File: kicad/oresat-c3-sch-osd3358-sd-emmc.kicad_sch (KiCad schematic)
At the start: 45 parts, among them J5 DM3BT-DSF-PEJS, U1 OSD3358-512M-BSM, U8 TCAN330, U9 EMMC+RESET+5.1-COMPATIBLE-BA

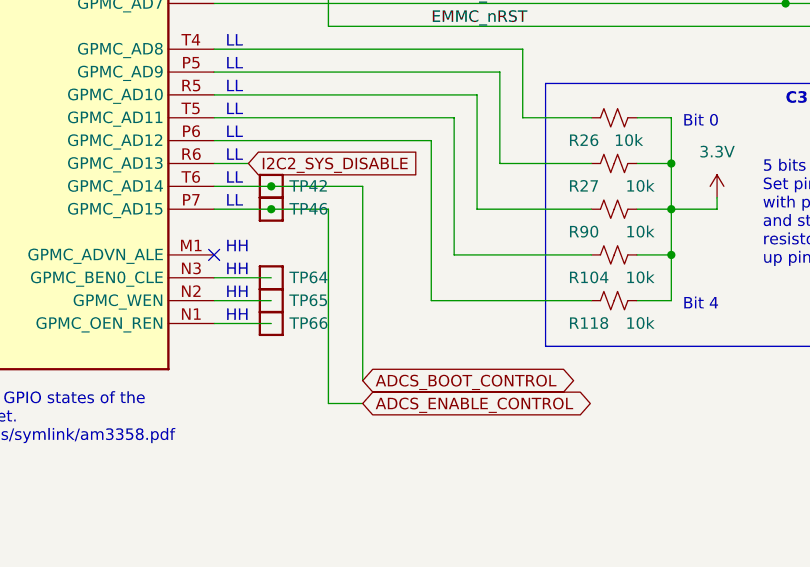
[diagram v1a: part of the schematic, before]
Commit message: - Locked CSKB Headers on PCB - Removed CAN1 from schematic - Removed ADCS boot enable from schematic - Removed unnecessary grounds from PCB
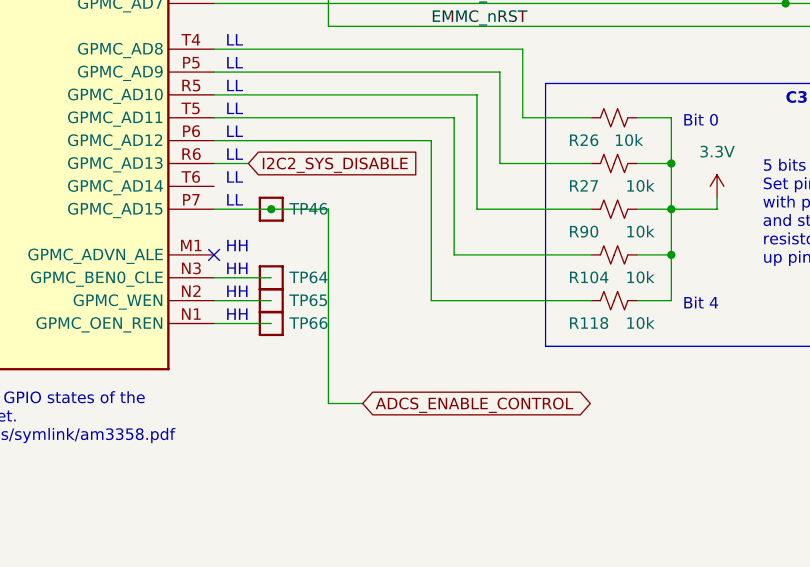
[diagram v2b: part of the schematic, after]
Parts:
- removed TP42: Test-Point, oresat-misc:TestPoint_Pad_D1.0mm, symbol oresat-misc:Test-Point-1mm-round
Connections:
- net ADCS_BOOT_CONTROL: no longer names the net of U1.T6 (GPMC_AD14)
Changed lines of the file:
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@@
 	)
 	(junction
-		(at 229.87 200.66)
-		(diameter 0)
-		(color 0 0 0 0)
-	)
-	(junction
 		(at 269.24 157.48)
 		(diameter 0)
@@
 	(wire
 		(pts
-			(xy 240.03 200.66) (xy 240.03 222.25)
-		)
-		(stroke
-			(width 0)
-			(type default)
-		)
-	)
-	(wire
-		(pts
 			(xy 269.24 104.14) (xy 278.13 104.14)
 		)
@@
 	(wire
 		(pts
-			(xy 240.03 200.66) (xy 229.87 200.66)
-		)
-		(stroke
-			(width 0)
-			(type default)
-		)
-	)
-	(wire
-		(pts
 			(xy 238.76 160.02) (xy 266.7 160.02)
 		)
@@
 	(wire
 		(pts
-			(xy 223.52 200.66) (xy 229.87 200.66)
-		)
-		(stroke
-			(width 0)
-			(type default)
-		)
-	)
-	(wire
-		(pts
 			(xy 270.51 193.04) (xy 274.32 193.04)
 		)
@@
 		)
 	)
-	(global_label "ADCS_BOOT_CONTROL"
-		(shape bidirectional)
-		(at 240.03 222.25 0)
-		(fields_autoplaced yes)
-		(effects
-			(font
-				(size 1.27 1.27)
-			)
-			(justify left)
-		)
-		(property "Intersheetrefs" "${INTERSHEET_REFS}"
-			(at 264.3256 222.25 0)
-			(effects
-				(font
-					(size 1.27 1.27)
-				)
-				(justify left)
-			)
-		)
-	)
 	(global_label "UART0_TX"
 		(shape input)
@@
 					(unit 1)
 				)
-			)
-		)
-	)
-	(symbol
-		(lib_id "oresat-misc:Test-Point-1mm-round")
-		(at 229.87 200.66 90)
-		(unit 1)
-		(exclude_from_sim no)
-		(in_bom yes)
-		(on_board yes)
-		(dnp no)
-		(property "Reference" "TP42"
-			(at 236.22 200.66 90)
-			(effects
-				(font
-					(size 1.27 1.27)
-				)
-				(justify left)
-			)
-		)
-		(property "Value" "Test-Point"
-			(at 227.33 200.66 0)
-			(effects
-				(font
-					(size 1.27 1.27)
-				)
-				(hide yes)
-			)
-		)
-		(property "Footprint" "oresat-misc:TestPoint_Pad_D1.0mm"
-			(at 219.71 200.66 0)
-			(effects
-				(font
-					(size 1.27 1.27)
-				)
-				(hide yes)
-			)
-		)
-		(property "Datasheet" ""
-			(at 229.87 200.66 0)
-			(effects
-				(font
-					(size 1.27 1.27)
-				)
-				(hide yes)
-			)
-		)
-		(property "Description" ""
-			(at 229.87 200.66 0)
-			(effects
-				(font
-					(size 1.27 1.27)
-				)
-				(hide yes)
-			)
-		)
-		(property "Part Page" ""
-			(at 229.87 200.66 0)
-			(effects
-				(font
-					(size 1.27 1.27)
-				)
-				(hide yes)
-			)
-		)
-		(property "Price" ""
-			(at 229.87 200.66 0)
-			(effects
-				(font
-					(size 1.27 1.27)
-				)
-				(hide yes)
-			)
-		)
-		(property "Total Price" ""
-			(at 229.87 200.66 0)
-			(effects
-				(font
-					(size 1.27 1.27)
-				)
-				(hide yes)
-			)
-		)
-		(pin "1"
-		)
-		(instances
-			(project "oresat-c3"
-				(path "/65d12cdd-c326-4033-9053-c59fa4e0b25e/f3d147ad-4cea-4d77-ae60-95882b03454e"
-					(reference "TP42")
-					(unit 1)
-				)

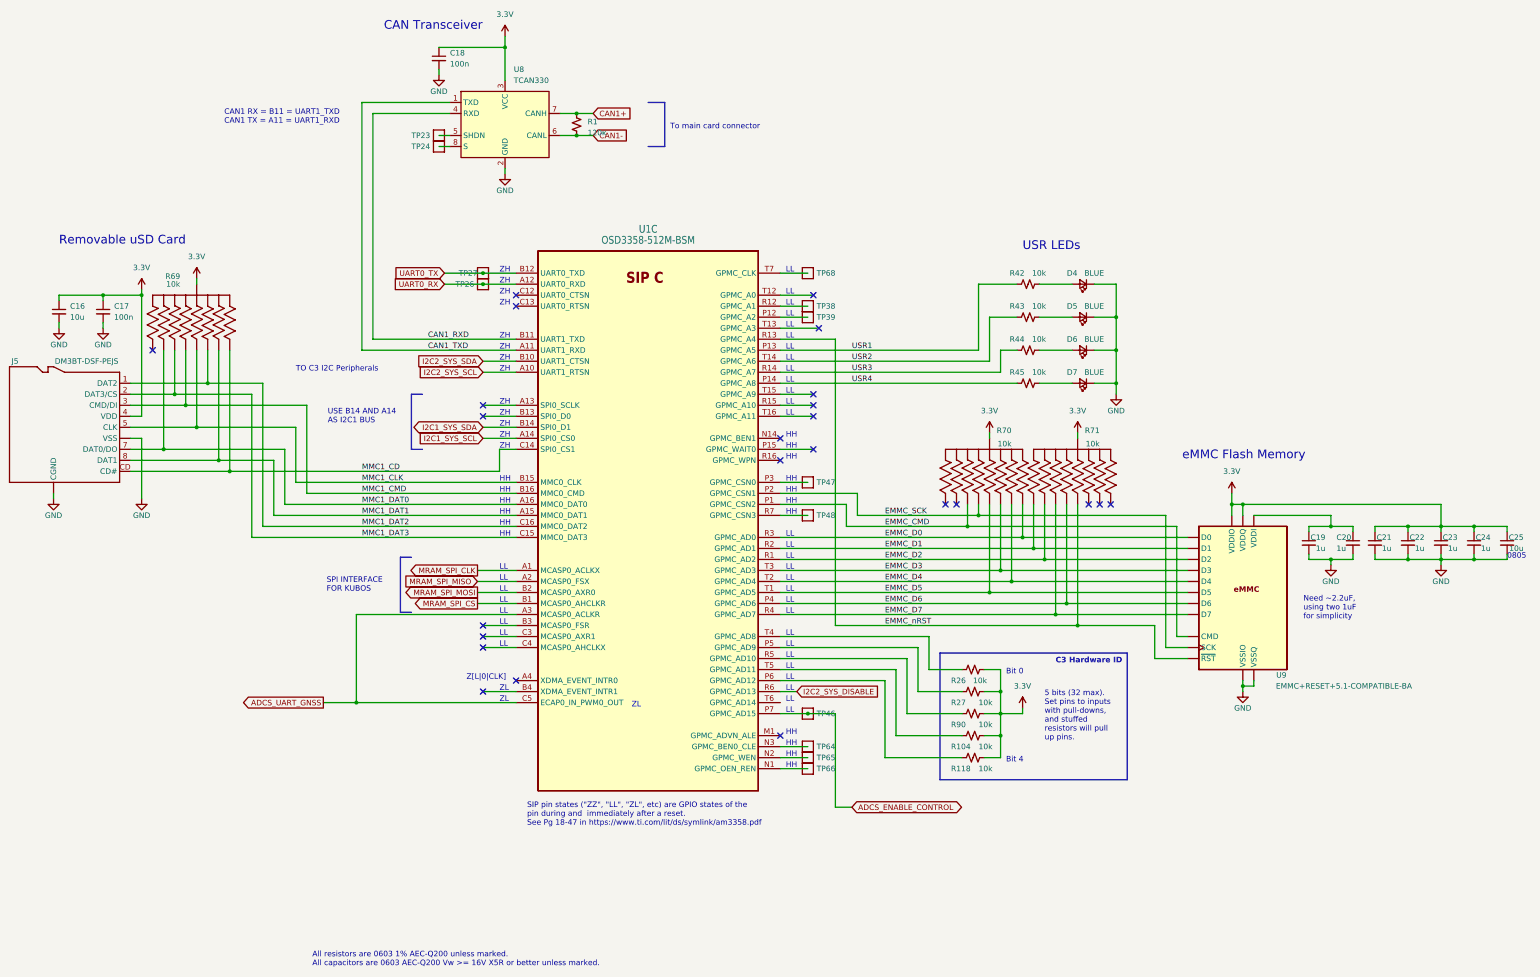
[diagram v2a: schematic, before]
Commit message: - Grounded FRAM Write protect permanently - Erased old CAN transceivers for unused bus - Fixed CAN termination resistor value to 120 ohm - Redid Clock skew for CAN lines - Removed UART0 from CSKB - Added second I2C buffer for I2C2 bus - Re-routed and placed all I2C bus components 	- Still need to route I2C sys disable, will do later after GPIOs since its lower prio - Added ADCS Enable pin components and routed everything
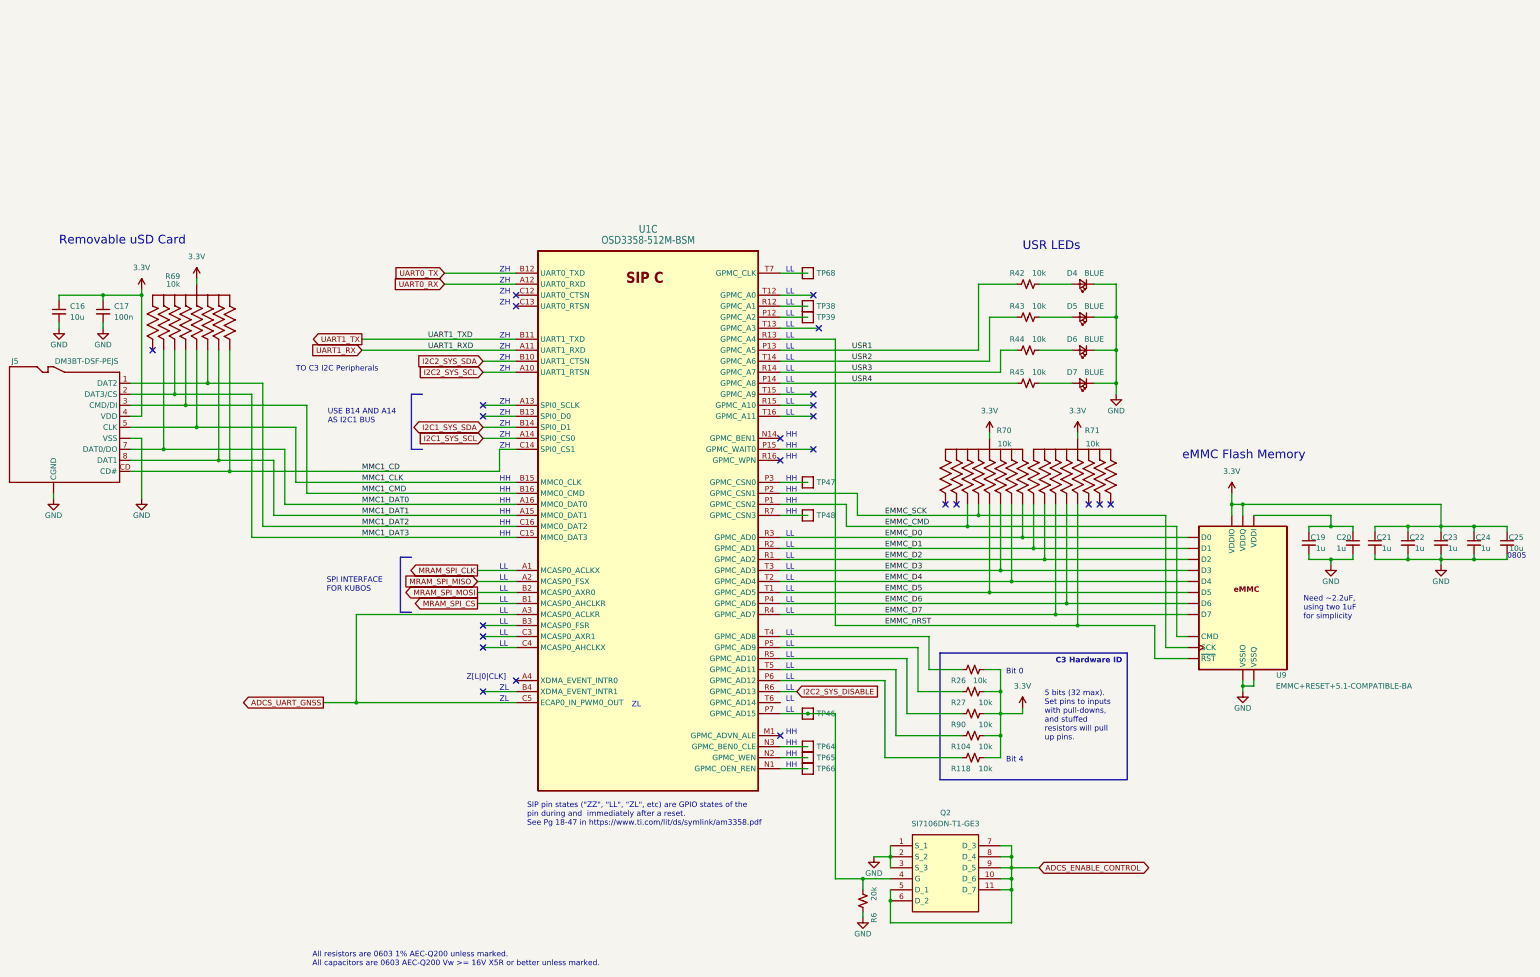
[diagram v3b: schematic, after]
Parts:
- removed C18: 100n, Capacitor_SMD:C_0603_1608Metric, symbol Device:C_Small
- removed R1: 120k, Resistor_SMD:R_0603_1608Metric, symbol Device:R_Small_US
- removed TP23, TP24, TP26, TP27: Test-Point, oresat-misc:TestPoint_Pad_D1.0mm, symbol oresat-misc:Test-Point-1mm-round
- removed U8: TCAN330, Package_TO_SOT_SMD:SOT-23-8, symbol Interface_CAN_LIN:TCAN330
- added Q2: SI7106DN-T1-GE3, SIS862DNT1GE3, symbol SI7106DN-T1-GE3:SI7106DN-T1-GE3
- added R6: 20k, Resistor_SMD:R_0603_1608Metric, symbol Device:R_Small_US
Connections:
- net ADCS_ENABLE_CONTROL: now also Q2.10 (D_6), Q2.11 (D_7), Q2.5 (D_1), Q2.6 (D_2), Q2.7 (D_3), Q2.8 (D_4), Q2.9 (D_5); no longer TP46.1, U1.P7 (GPMC_AD15)
- net GND: now also Q2.1 (S_1), Q2.2 (S_2), Q2.3 (S_3), R6.2
- net CAN1_RXD renamed UART1_TX
- net CAN1_TXD renamed UART1_RX
- new net: Q2.4 (G), R6.1, TP46.1, U1.P7 (GPMC_AD15)
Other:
- note removed: "CAN Transceiver"
- note removed: "CAN1 RX = B11 = UART1_TXD CAN1 TX = A11 = UART1_RXD"
- note removed: "To main card connector"

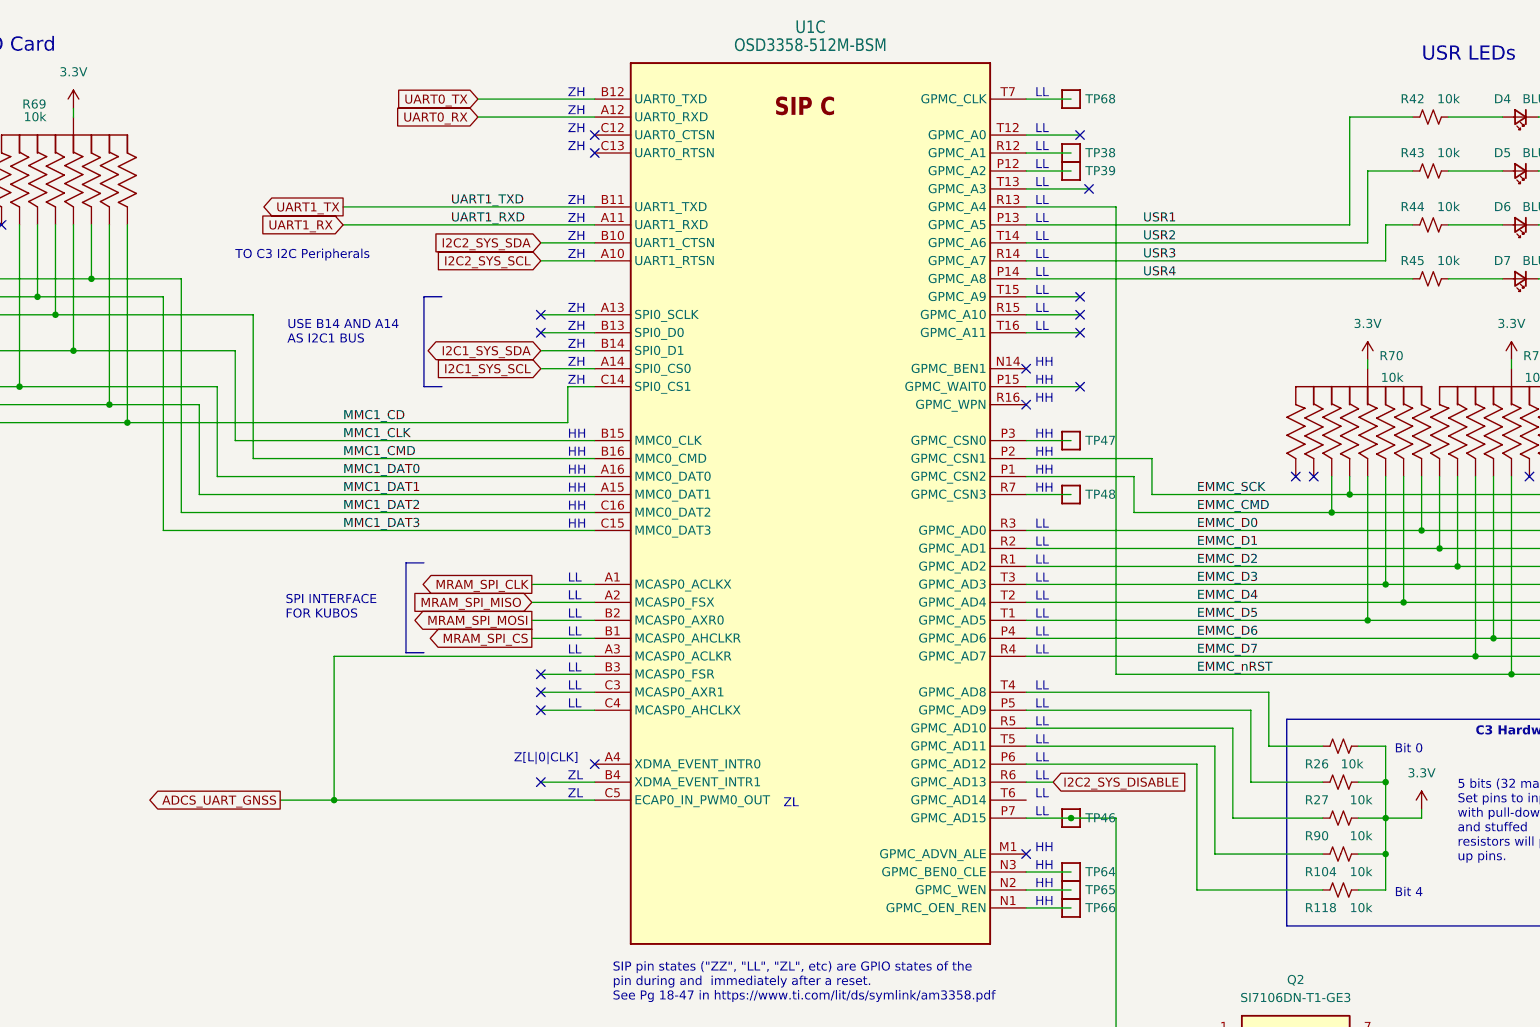
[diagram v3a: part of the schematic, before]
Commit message: - Labelled GPIOs and UART lines to processor pins - Routed UART lines - Routed GPIO Lines - Refilled zones - Added via fencing back in - Board should be ready to be reviewed now
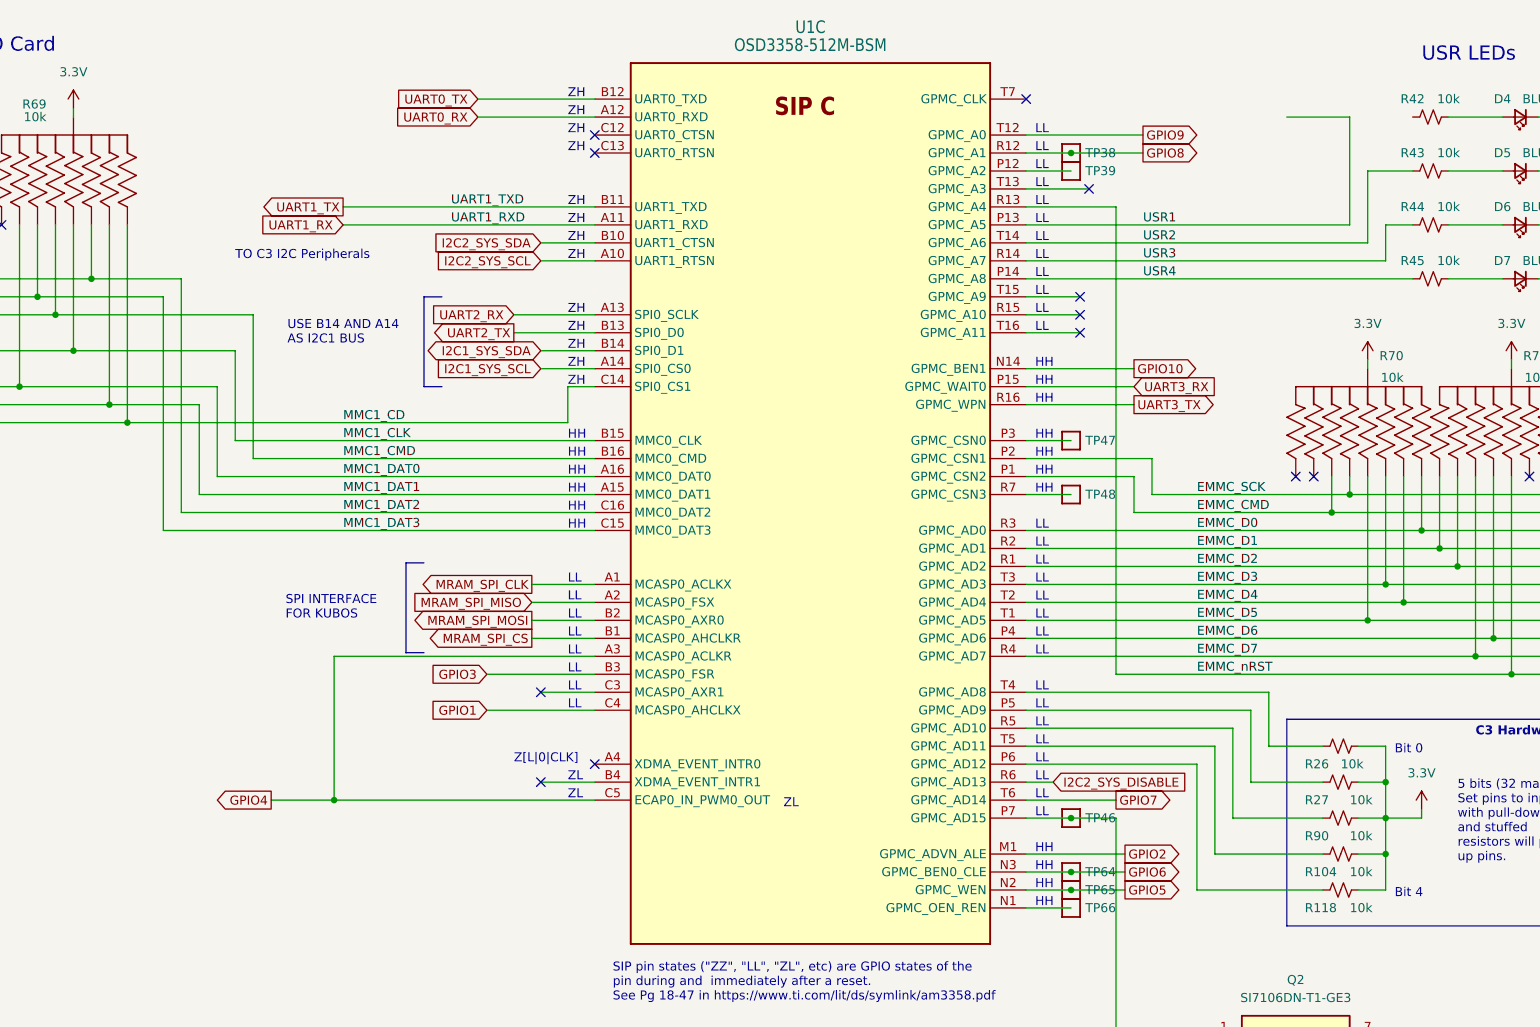
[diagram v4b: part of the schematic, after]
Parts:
- removed TP68: Test-Point, oresat-misc:TestPoint_Pad_D1.0mm, symbol oresat-misc:Test-Point-1mm-round
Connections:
- net USR1: no longer R42.1
- net GPIO8: now reaches TP38.1, U1.R12 (GPMC_A1)
- net UART2_RX: now reaches U1.A13 (SPI0_SCLK)
- net UART2_TX: now reaches U1.B13 (SPI0_D0)
- net GPIO3: now reaches U1.B3 (MCASP0_FSR)
- net GPIO1: now reaches U1.C4 (MCASP0_AHCLKX)
- net GPIO2: now reaches U1.M1 (GPMC_ADVN_ALE)
- net GPIO10: now reaches U1.N14 (GPMC_BEN1)
- net GPIO5: now reaches TP65.1, U1.N2 (GPMC_WEN)
- net GPIO6: now reaches TP64.1, U1.N3 (GPMC_BEN0_CLE)
- net UART3_RX: now reaches U1.P15 (GPMC_WAIT0)
- net UART3_TX: now reaches U1.R16 (GPMC_WPN)
- net GPIO9: now reaches U1.T12 (GPMC_A0)
- net GPIO7: now reaches U1.T6 (GPMC_AD14)
- net ADCS_UART_GNSS renamed GPIO4
- no-connect marks 24 -> 16

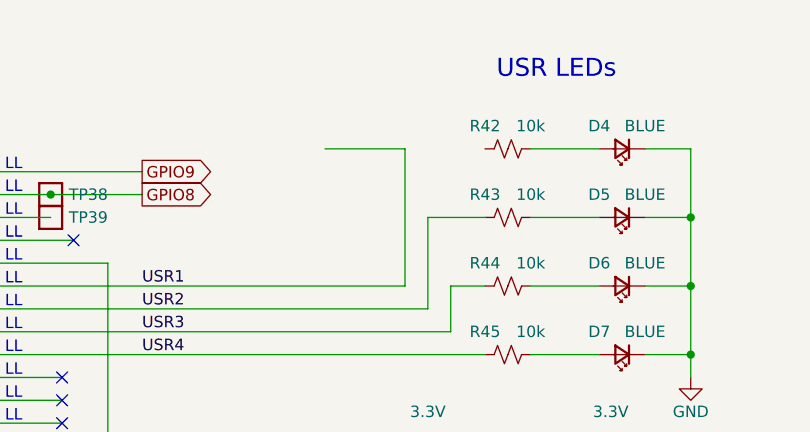
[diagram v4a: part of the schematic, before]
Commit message: OBC review session changes
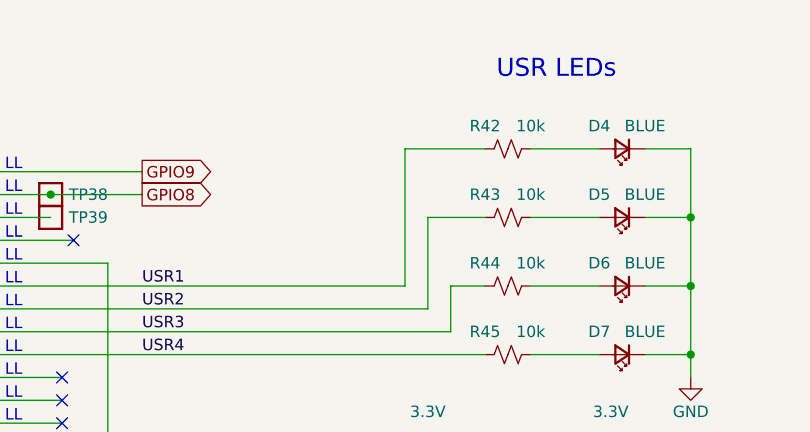
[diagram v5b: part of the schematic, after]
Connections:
- net USR1: now also R42.1
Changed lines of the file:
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@@
-	(wire
-		(pts
-			(xy 269.24 104.14) (xy 260.35 104.14)
-		)
-		(stroke
-			(width 0)
-			(type default)
-		)
-	)
 	(wire
 		(pts
@@
 		)
 		(stroke
+			(width 0)
+			(type default)
+		)
+	)
+	(wire
+		(pts
+			(xy 269.24 104.14) (xy 278.13 104.14)
+		)
+		(stroke
